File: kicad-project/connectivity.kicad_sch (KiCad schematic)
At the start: 21 parts, among them J5 Compass, J6 Accelerometer, J7 OLED, Q1 3LP01M, Q2 PDTC114Y, Q3 BC846A, Q4 BC846A, Q5 BC846A, U4 PAM-7Q-0

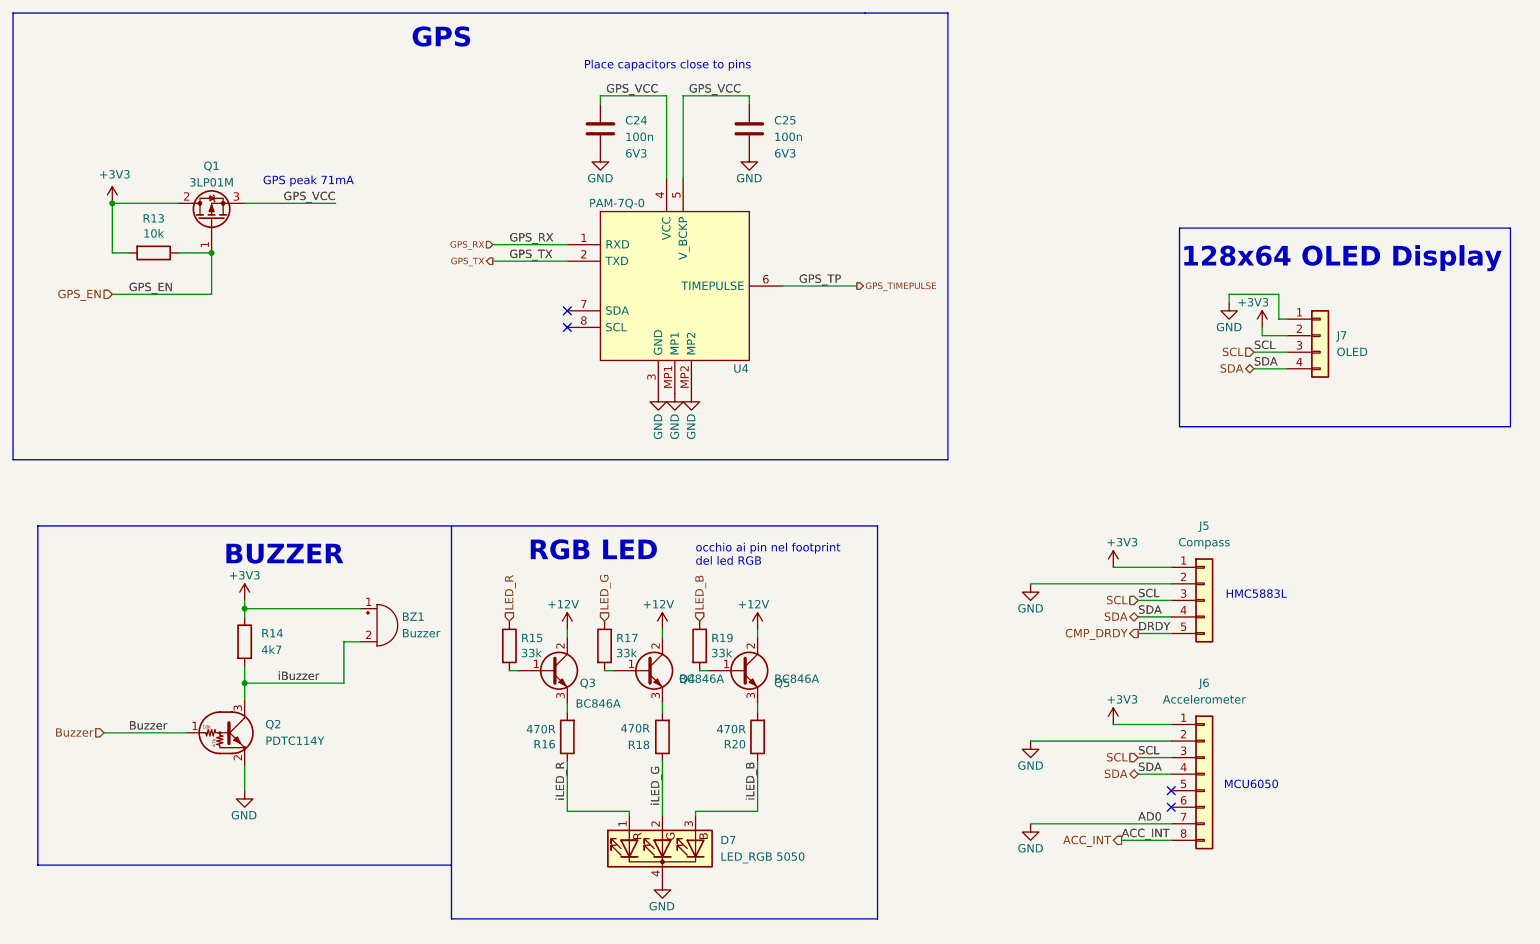
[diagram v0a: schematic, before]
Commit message: hw: changes for the simia
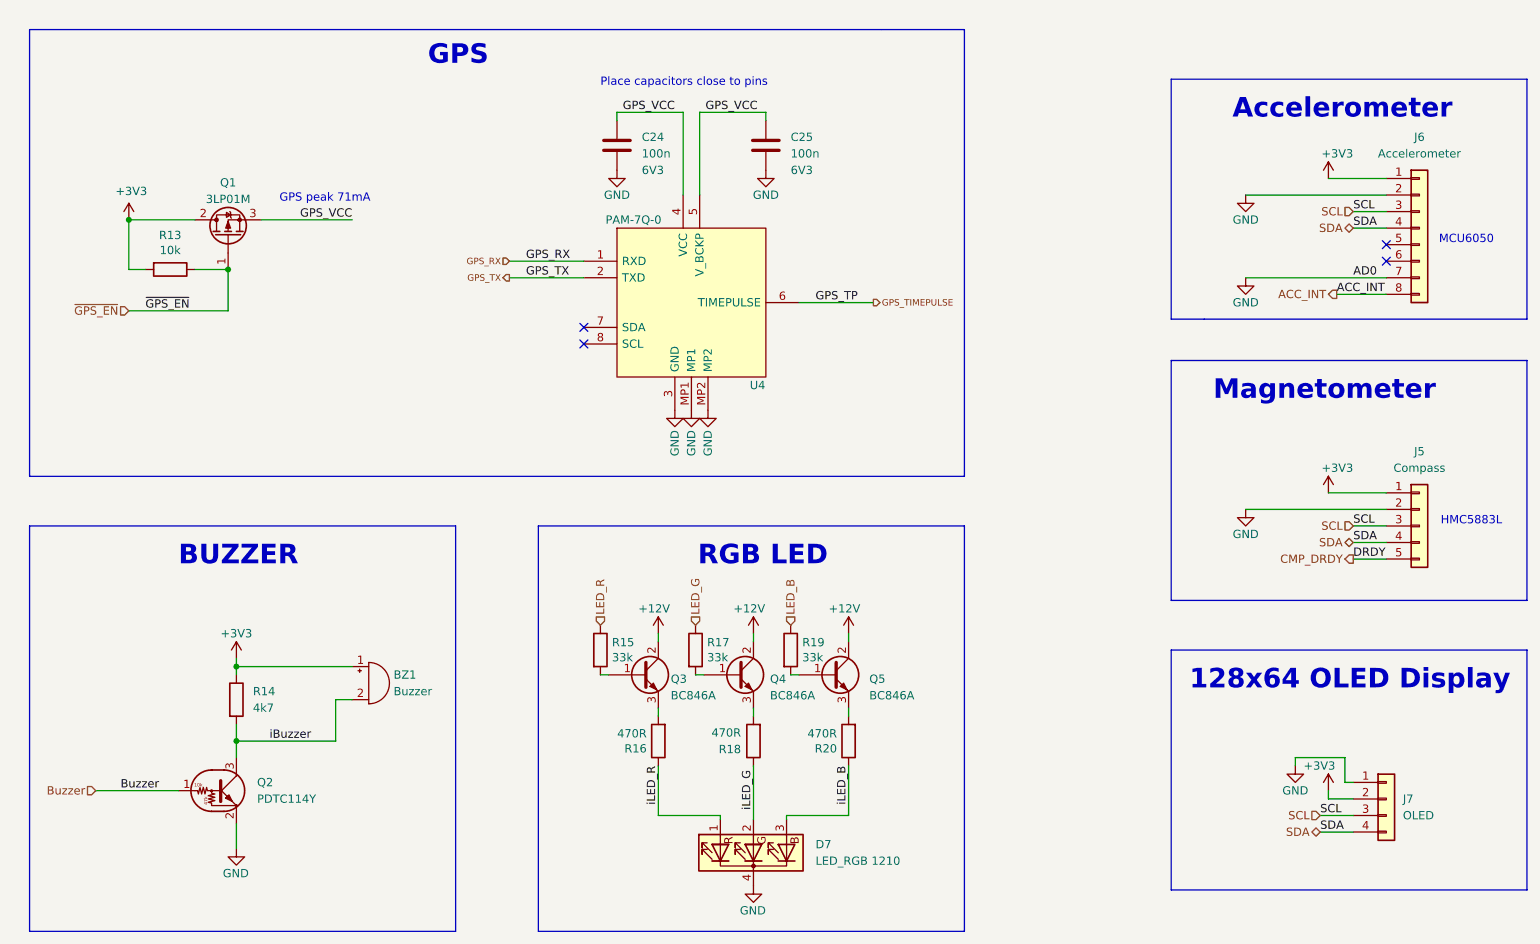
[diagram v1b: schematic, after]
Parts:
- D7: value LED_RGB 5050 -> LED_RGB 1210
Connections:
- net GPS_EN renamed ~{GPS_EN}
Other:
- note added: "Accelerometer"
- note added: "Magnetometer"
- note removed: "occhio ai pin nel footprint del led RGB"
- moved on the sheet: BZ1, C24, C25, D7, J5, J6, J7, Q1, Q2, Q3, Q4, Q5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
